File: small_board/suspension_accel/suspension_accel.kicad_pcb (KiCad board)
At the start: 4 copper layers, 20.6 x 74 mm, 48 parts, among them IC1 TJA1050T_CM,118, IC2 AMS1117-3.3, IC3 SN74LVC1T45DCKR, IC4 ESP32-S3-MINI-1-N8, IC5 ADS1220IPWR, IC6 TLV75533PDBVR, IC7 SN74LVC1T45DCKR, J1 OSTTE040104, J2 BM04B-GVHS-TB_LF__SN_

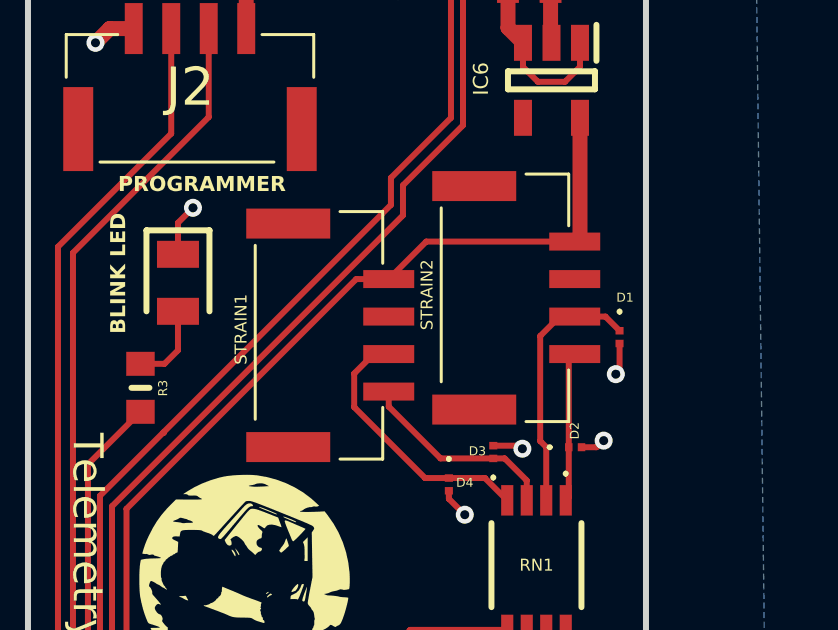
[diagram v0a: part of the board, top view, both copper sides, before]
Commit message: prepared for manufacturing first iter
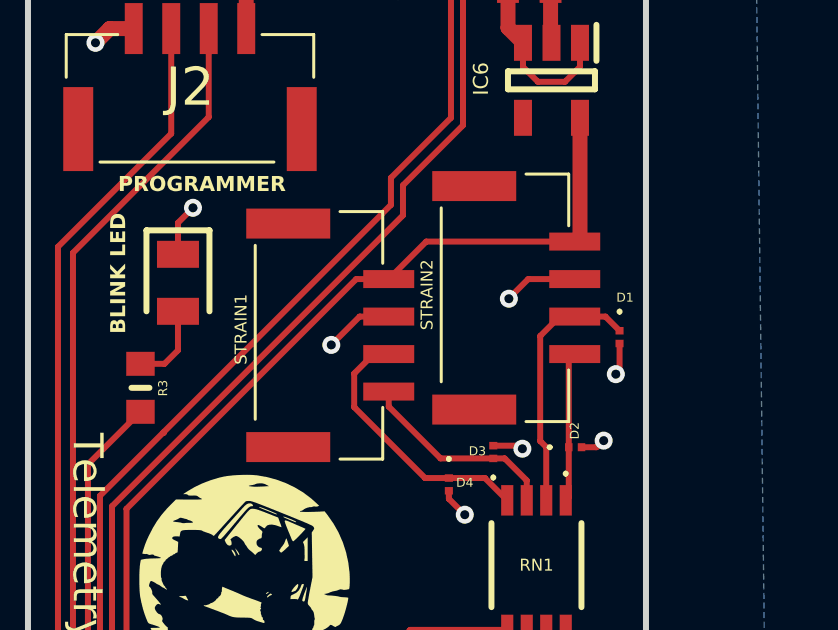
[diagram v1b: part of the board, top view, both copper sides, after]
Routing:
- net GND: track 40.0 -> 44.8 mm, vias 42 -> 44
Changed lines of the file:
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@@
 			)
 		)
+		(model "/home/marcus/Desktop/telemetry_pcb_1/small_board/components/LIB_D5V0F1U2LP-7B/D5V0F1U2LP-7B/3D/D5V0F1U2LP-7B.stp"
+			(offset
+				(xyz 0 0 0)
+			)
+			(scale
+				(xyz 1 1 1)
+			)
+			(rotate
+				(xyz -90 -0 -0)
+			)
+		)
 	)
 	(footprint "MountingHole:MountingHole_2.2mm_M2"
@@
 			)
 		)
+		(model "/home/marcus/Desktop/telemetry_pcb_1/small_board/components/LIB_RCLAMP3521ZATFT/RCLAMP3521ZATFT/3D/RCLAMP3521ZATFT.stp"
+			(offset
+				(xyz 0 0 0)
+			)
+			(scale
+				(xyz 1 1 1)
+			)
+			(rotate
+				(xyz 0 0 0)
+			)
+		)
 	)
 	(footprint "Library:RESC1608X60N"
@@
 			)
 		)
+		(model "/home/marcus/Desktop/telemetry_pcb_1/small_board/components/LIB_RCLAMP3521ZATFT/RCLAMP3521ZATFT/3D/RCLAMP3521ZATFT.stp"
+			(offset
+				(xyz 0 0 0)
+			)
+			(scale
+				(xyz 1 1 1)
+			)
+			(rotate
+				(xyz 0 0 0)
+			)
+		)
 	)
 	(footprint "Library:canada"
@@
 			(at -0.13716 -13.4493 0)
 			(layer "B.SilkS")
+			(hide yes)
 			(effects
 				(font
@@
 	)
 	(segment
+		(start 33.055 54.625)
+		(end 32.11 55.57)
+		(width 0.2)
+		(layer "F.Cu")
+		(net 2)
+	)
+	(segment
 		(start 34 42.45)
 		(end 34 43.5)
@@
 	)
 	(segment
+		(start 34.025 54.625)
+		(end 33.055 54.625)
+		(width 0.2)
+		(layer "F.Cu")
+		(net 2)
+	)
+	(segment
 		(start 38.378 58.928)
 		(end 38.48 59.03)
@@
 	)
 	(segment
+		(start 40.225 53.375)
+		(end 38.675 53.375)
+		(width 0.2)
+		(layer "F.Cu")
+		(net 2)
+	)
+	(segment
 		(start 38.65 77.35)
 		(end 38 78)
@@
 	)
 	(segment
+		(start 38.675 53.375)
+		(end 38 54.05)
+		(width 0.2)
+		(layer "F.Cu")
+		(net 2)
+	)
+	(segment
 		(start 27.75 32.75)
 		(end 28.28 33.28)
@@
 		(net 2)
 	)
+	(segment
+		(start 32.11 55.57)
+		(end 32.08 55.6)
+		(width 0.2)
+		(layer "F.Cu")
+		(net 2)
+	)
+	(via
+		(at 32.11 55.57)
+		(size 0.6)
+		(drill 0.3)
+		(layers "F.Cu" "B.Cu")
+		(net 2)
+	)
 	(via
 		(at 35 78)
@@
 	)
 	(via
+		(at 38.03 54.03)
+		(size 0.6)
+		(drill 0.3)
+		(layers "F.Cu" "B.Cu")
+		(net 2)
+	)
+	(via
 		(at 39 72)
 		(size 0.6)
@@
 		(hatch edge 0.5)
 		(priority 3)
-		(connect_pads
+		(connect_pads yes
 			(clearance 0)
 		)
